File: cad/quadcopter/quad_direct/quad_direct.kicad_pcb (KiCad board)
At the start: 2 copper layers, 24.9 x 40.4 mm, 18 parts, among them SW1 SW_Push, SW2 SW_Push, U1 4pin_header, U2 esp32c3_boardout, U4 3pin_header

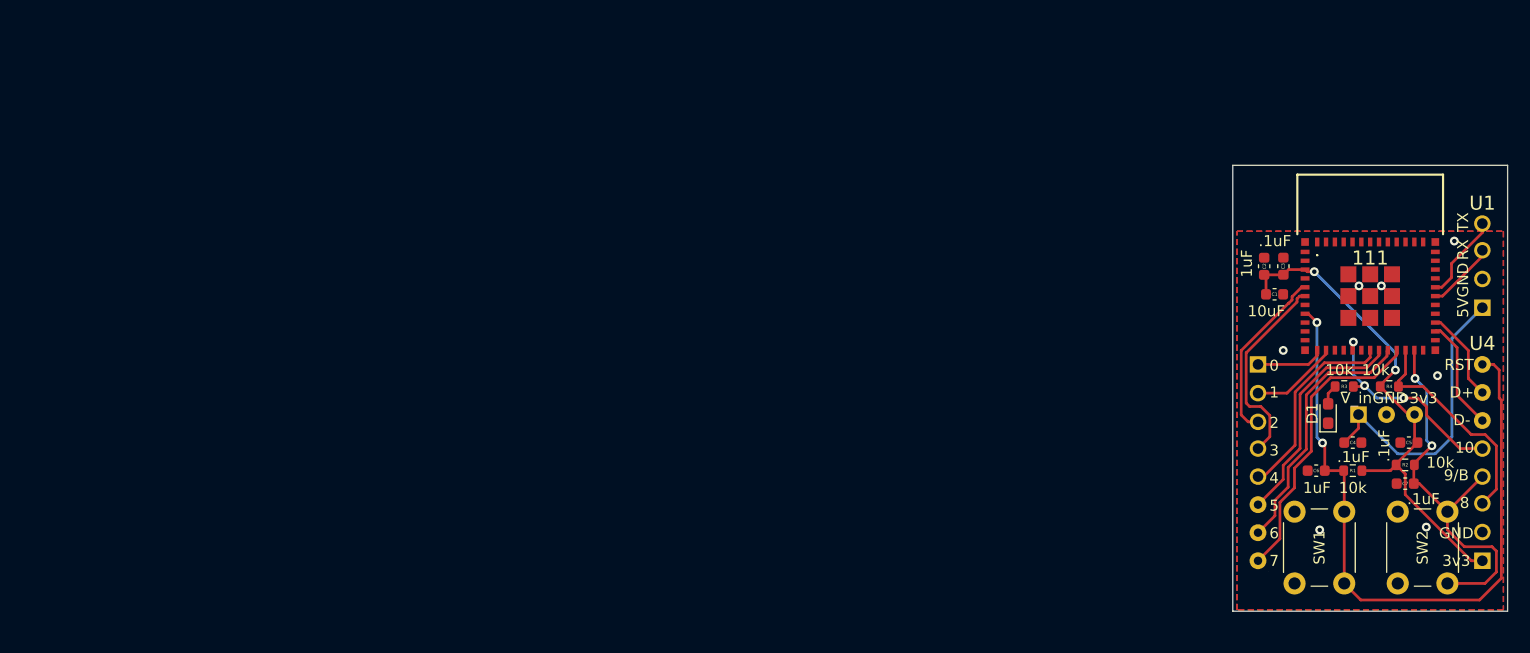
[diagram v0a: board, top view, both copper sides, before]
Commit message: boardy boards
Signed-off-by: Andrew Wock <ajwock@gmail.com>
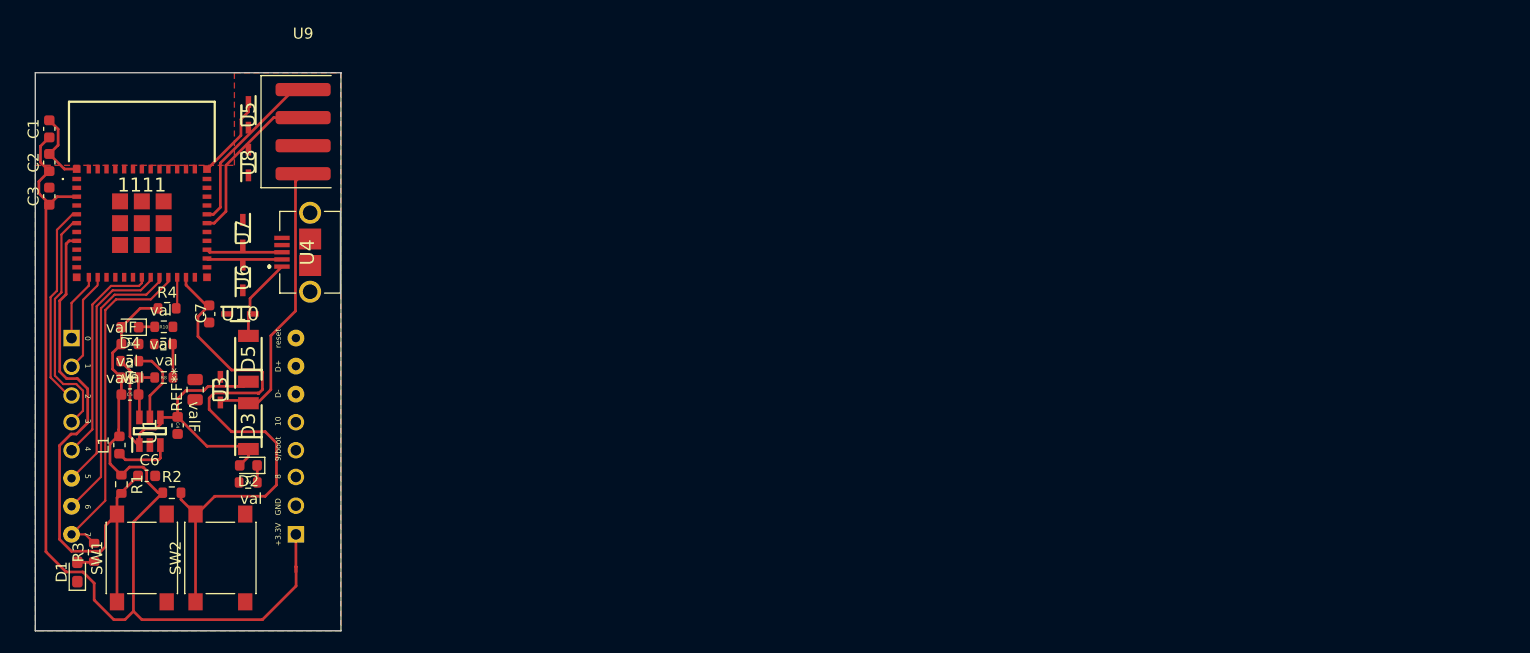
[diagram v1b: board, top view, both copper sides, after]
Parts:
- removed 111: ESP32-C3-MINI-1-H4X, Imported:ESP32C3MINI1H4X
- added 1111: ESP32-C3-MINI-1-H4X, Imported:ESP32C3MINI1H4X, F.Cu at (53.8, 29.0)
- added C8: 22uF, Imported:0603_cap, F.Cu at (52.0, 42.6)
- added D2: LED, LED_SMD:LED_0603_1608Metric, F.Cu at (63.5, 53.6)
- added D3: D_Schottky, Imported:SM6F22AY, F.Cu at (63.5, 50.0)
- added D4: LED, LED_SMD:LED_0603_1608Metric, F.Cu at (52.8, 41.1)
- added D5: D_Schottky, Imported:SM6F22AY, F.Cu at (63.5, 43.9)
- added L1: L, Inductor_SMD:L_0603_1608Metric, F.Cu at (51.8, 51.7)
- added R10: 4.7k, Imported:0603_resistor, F.Cu at (55.8, 41.1)
- added R5: 6.8k, Imported:0603_resistor, F.Cu at (63.5, 55.1)
- added R6: 470k, Imported:0603_resistor, F.Cu at (52.8, 44.1)
- added R7: 220k, Imported:0603_resistor, F.Cu at (52.8, 45.7)
- added R8: 47k, Imported:0603_resistor, F.Cu at (55.8, 45.7)
- added R9: 2.2k, Imported:0603_resistor, F.Cu at (55.8, 42.6)
- added REF**: 0_ohm, Imported:0_ohm, F.Cu at (58.7, 46.7)
- added U10: SD03C-7, Imported:SOD2513X120N, F.Cu at (62.7, 39.9)
- added U3: SD03C-7, Imported:SOD2513X120N, F.Cu at (61.0, 46.7)
- added U5: SD03C-7, Imported:SOD2513X120N, F.Cu at (63.5, 21.8)
- added U6: SD03C-7, Imported:SOD2513X120N, F.Cu at (63.0, 36.6)
- added U7: SD03C-7, Imported:SOD2513X120N, F.Cu at (63.0, 32.5)
- added U8: SD03C-7, Imported:SOD2513X120N, F.Cu at (63.5, 26.2)
- added U9: 4pin_header, Imported:4-rightangle-smt, F.Cu at (68.5, 27.2)
- C4: value .1u -> 10uF; footprint Capacitor_SMD:C_0603_1608Metric -> Imported:0603_cap
- C5: value .1u -> 10pf; footprint Capacitor_SMD:C_0603_1608Metric -> Imported:0603_cap
- SW1, SW2: footprint Button_Switch_THT:SW_PUSH_6mm -> Button_Switch_SMD:SW_Push_1P1T_NO_6x6mm_H9.5mm
- U1: value 4pin_header -> TPS62A02APDDCR; footprint Imported:4-bb -> Imported:SOT95P280X110-6N
- U4: value 3pin_header -> USB3090-30-A; footprint Imported:3-bb -> Imported:USB309030A
- moved U1 121.2 mm to (54.6, 50.5)
- moved C5 116.7 mm to (52.0, 47.2)
- moved R3 114.2 mm to (49.5, 61.5), turned to 90 degrees
- moved D1 114.2 mm to (48.0, 63.2)
- moved C1 112.0 mm to (45.5, 23.1), turned to 90 degrees
- moved C3 112.0 mm to (45.5, 29.2)
- moved R2 111.7 mm to (56.6, 56.1)
- moved R1 111.5 mm to (52.0, 55.3), turned to -90 degrees
- moved SW2 111.2 mm to (61.0, 62.0), turned to 90 degrees
- moved R4 110.9 mm to (56.1, 39.4)
- moved C2 110.4 mm to (45.5, 26.2)
- moved C7 109.4 mm to (59.9, 39.9), turned to 90 degrees
- moved SW1 109.0 mm to (53.8, 62.0), turned to 90 degrees
- moved U2 107.5 mm to (44.9, 61.1)
- moved C4 106.5 mm to (57.1, 49.2), turned to -90 degrees
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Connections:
- C1 pad 1: +3V3 -> +3.3V
- C2 pad 1: +3V3 -> +3.3V
- C3 pad 1: +3V3 -> +3.3V
- C4 pad 1: +5V -> VBUS
- C5 pad 1: GND -> +3.3V
- C5 pad 2: +3V3 -> Net-(C5-Pad2)
- R1 pad 1: +3V3 -> +3.3V
- R2 pad 1: +3V3 -> +3.3V
- R3 pad 2: IO10 -> IO7
- R4 pad 1: +3V3 -> +3.3V
- U1 pad 1: +5V -> VBUS
- U1 pad 3: UART_RX -> Net-(L1-Pad1)
- U1 pad 4: UART_TX -> VBUS
- U2 pad 10: IO19_USB_D+ -> unconnected-(U2-Pad10)
- U2 pad 11: IO18_USB_D- -> unconnected-(U2-Pad11)
- U2 pad 12: IO10 -> unconnected-(U2-Pad12)
- U2 pad 13: IO9_BOOT -> unconnected-(U2-Pad13)
- U2 pad 14: IO8 -> unconnected-(U2-Pad14)
- U2 pad 16: +3V3 -> +3.3V
- U2 pad 9: RESET -> unconnected-(U2-Pad9)
- U4 pad 1: +5V -> Net-(D5-Pad2)
- U4 pad 2: GND -> IO18_USB_D-
- U4 pad 3: +3V3 -> IO19_USB_D+
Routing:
- net +3.3V: track 0.00 -> 111.6 mm
- net +3V3: track 46.1 -> 0.00 mm, vias 2 -> 0
- net VBUS: track 0.00 -> 32.1 mm
- net +5V: track 26.5 -> 0.00 mm
- net Net-(D3-Pad2): track 0.00 -> 26.5 mm
- net IO10: track 19.7 -> 0.00 mm, vias 3 -> 0
- net IO8: track 20.4 -> 2.46 mm
- net IO9_BOOT: track 35.6 -> 51.5 mm, vias 2 -> 0
- net GND: track 0.00 -> 14.4 mm, vias 7 -> 0
- net RESET: track 63.4 -> 51.4 mm, vias 2 -> 0
- net UART_RX: track 6.30 -> 15.1 mm
- net UART_TX: track 7.88 -> 15.7 mm
- net Net-(D5-Pad2): track 0.00 -> 7.54 mm
- net Net-(R6-Pad1): track 0.00 -> 7.16 mm
- net Net-(L1-Pad1): track 0.00 -> 5.18 mm
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- removed copper zone on B.Cu, net GND
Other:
- board size 24.9 x 40.4 mm -> 27.7 x 50.5 mm
